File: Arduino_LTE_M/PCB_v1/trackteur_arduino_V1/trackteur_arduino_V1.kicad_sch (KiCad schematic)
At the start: 17 parts, among them J1 rPi_HDR, J2 DC/DC, J3 BATT_CAR, J4 MicroSD_Breakout, Q1 2N3904, U1 LD1117S33TR_SOT223

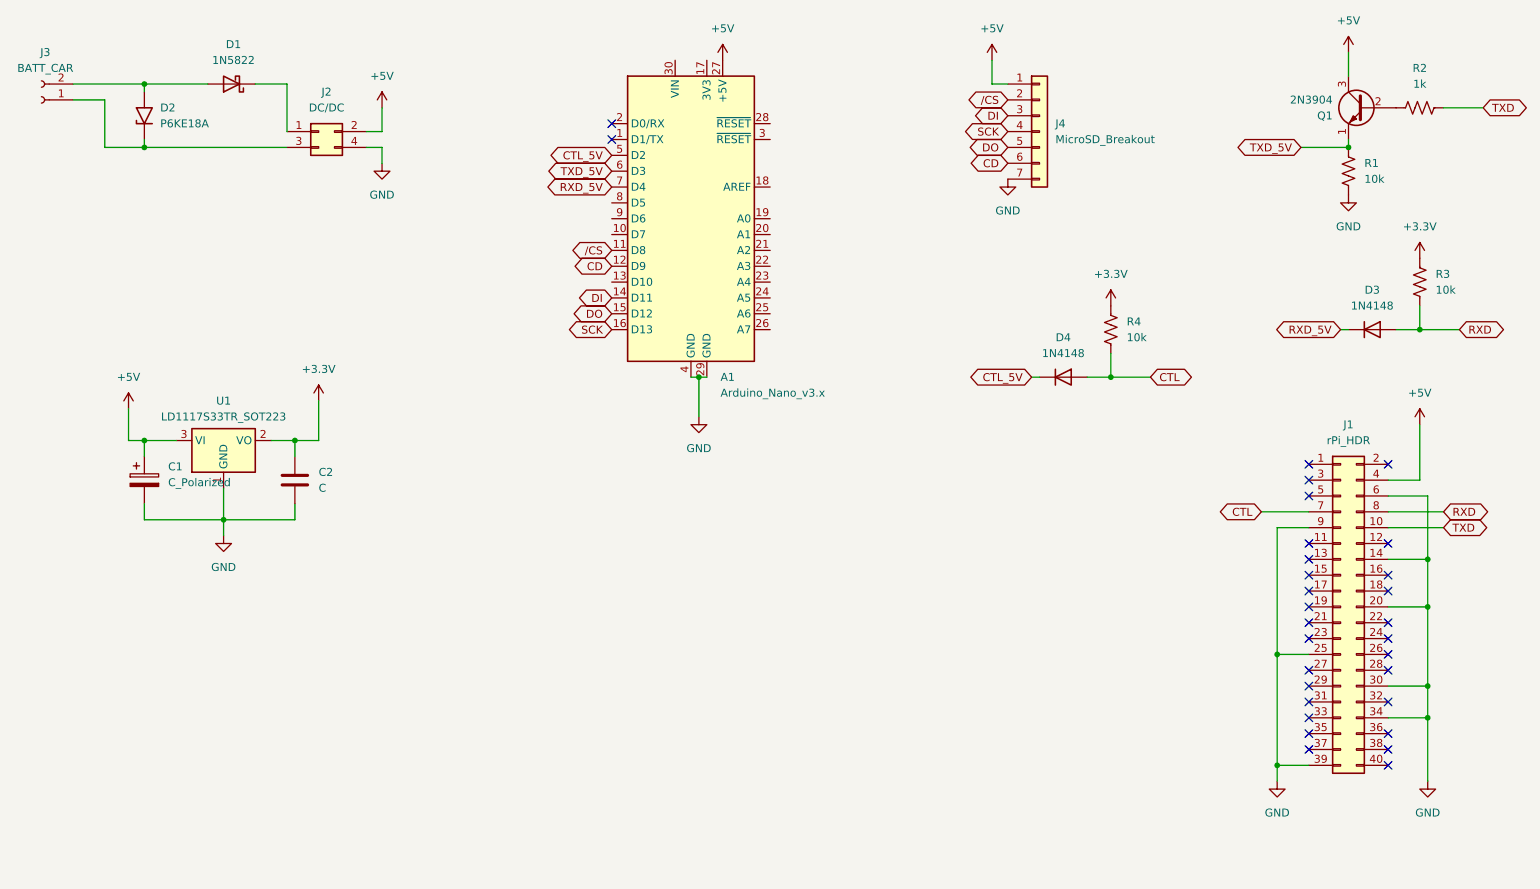
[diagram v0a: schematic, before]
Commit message: update PCB
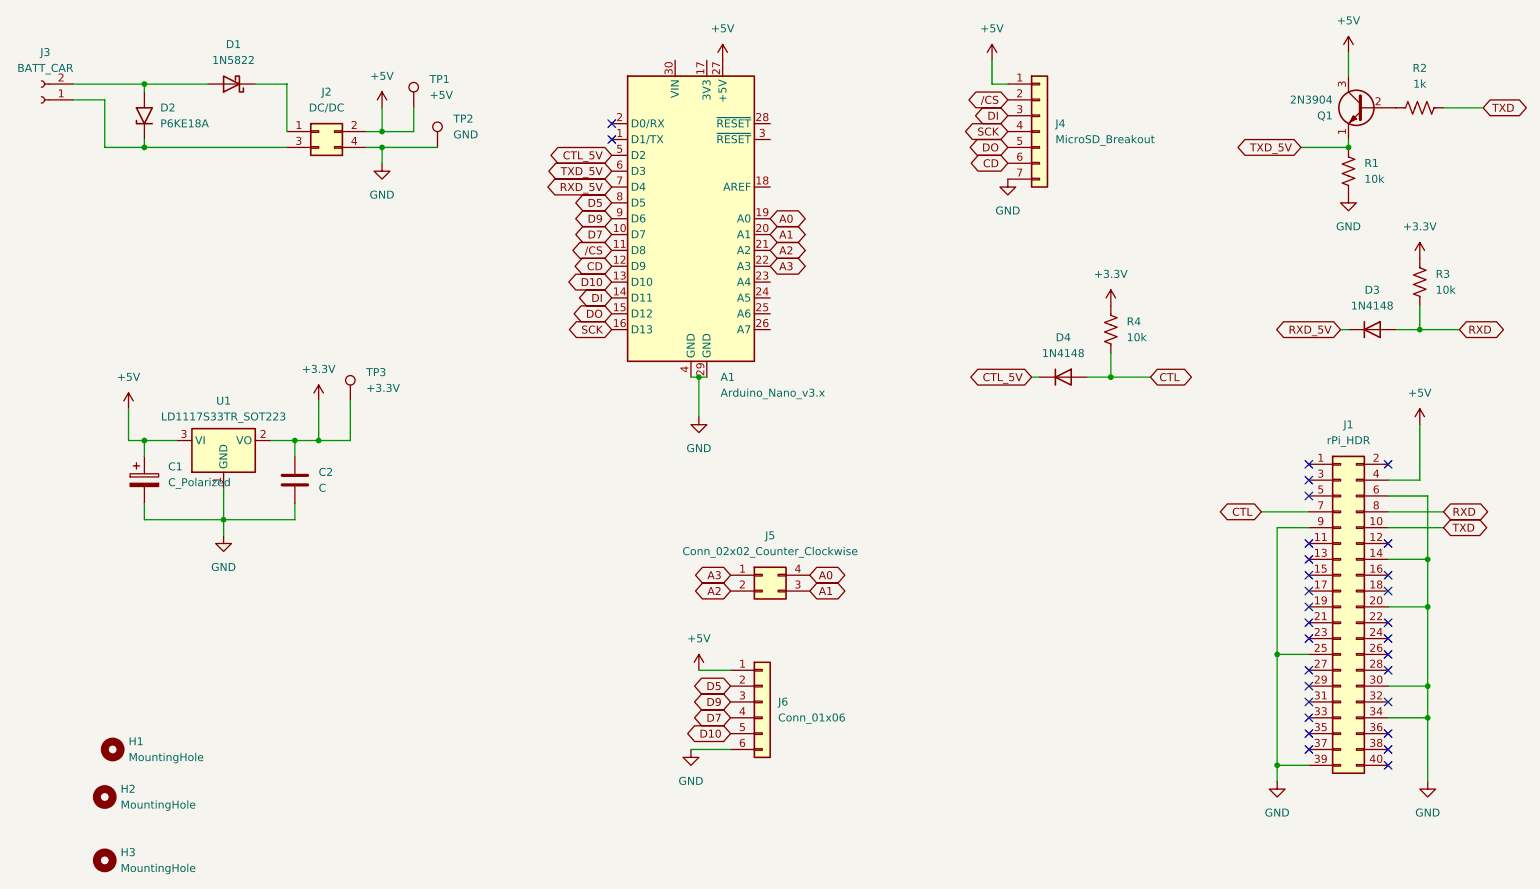
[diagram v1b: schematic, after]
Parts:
- added H1, H2, H3: MountingHole, MountingHole:MountingHole_2.7mm_M2.5, symbol Mechanical:MountingHole
- added J5: Conn_02x02_Counter_Clockwise, Connector_PinHeader_2.54mm:PinHeader_2x02_P2.54mm_Vertical, symbol Connector_Generic:Conn_02x02_Counter_Clockwise
- added J6: Conn_01x06, Connector_PinHeader_2.54mm:PinHeader_1x06_P2.54mm_Vertical, symbol Connector_Generic:Conn_01x06
- added TP1: +5V, Connector_PinHeader_2.54mm:PinHeader_1x01_P2.54mm_Vertical, symbol Connector:TestPoint
- added TP2: GND, Connector_PinHeader_2.54mm:PinHeader_1x01_P2.54mm_Vertical, symbol Connector:TestPoint
- added TP3: +3.3V, Connector_PinHeader_2.54mm:PinHeader_1x01_P2.54mm_Vertical, symbol Connector:TestPoint
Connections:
- net +3.3V: now also TP3.1
- net +5V: now also J6.1 (Pin_1), TP1.1
- net GND: now also J6.6 (Pin_6), TP2.1
- net D7: now reaches A1.10 (D7)
- net D7: now also J6.4 (Pin_4)
- net D10: now reaches A1.13 (D10)
- net D10: now also J6.5 (Pin_5)
- net A0: now reaches A1.19 (A0)
- net A0: now also J5.4 (Pin_4)
- net A1: now reaches A1.20 (A1)
- net A1: now also J5.3 (Pin_3)
- net A2: now reaches A1.21 (A2)
- net A2: now also J5.2 (Pin_2)
- net A3: now reaches A1.22 (A3)
- net A3: now also J5.1 (Pin_1)
- net D5: now reaches A1.8 (D5)
- net D5: now also J6.2 (Pin_2)
- net D9: now reaches A1.9 (D6)
- net D9: now also J6.3 (Pin_3)

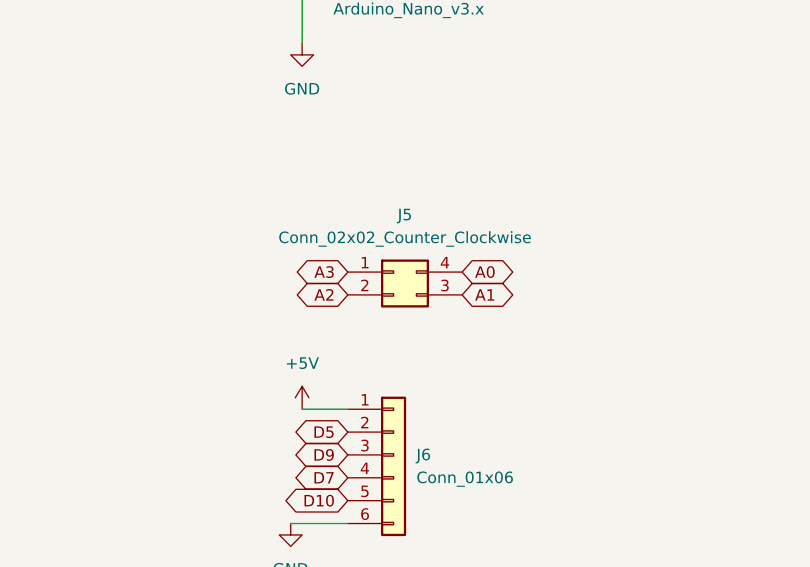
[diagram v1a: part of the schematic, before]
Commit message: Fichiers de fabrication
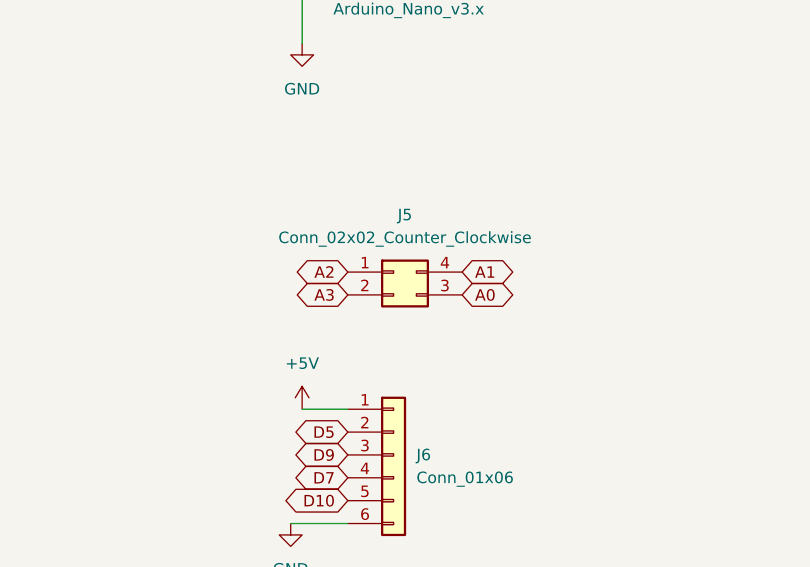
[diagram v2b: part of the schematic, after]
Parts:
- J3: footprint Connector_Wire:SolderWire-0.75sqmm_1x02_P7mm_D1.25mm_OD3.5mm -> Connector_Wire:SolderWire-2.5sqmm_1x02_P7.2mm_D2.4mm_OD3.6mm
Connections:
- net A0: now also J5.3 (Pin_3); no longer J5.4 (Pin_4)
- net A1: now also J5.4 (Pin_4); no longer J5.3 (Pin_3)
- net A2: now also J5.1 (Pin_1); no longer J5.2 (Pin_2)
- net A3: now also J5.2 (Pin_2); no longer J5.1 (Pin_1)
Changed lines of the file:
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@@
     )
   )
-  (global_label "A2" (shape bidirectional) (at 137.16 120.65 180) (fields_autoplaced)
+  (global_label "A3" (shape bidirectional) (at 137.16 120.65 180) (fields_autoplaced)
     (effects (font (size 1.27 1.27)) (justify right))
     (property "Intersheetrefs" "${INTERSHEET_REFS}" (at 130.7654 120.65 0)
@@
     )
   )
-  (global_label "A3" (shape bidirectional) (at 137.16 118.11 180) (fields_autoplaced)
+  (global_label "A2" (shape bidirectional) (at 137.16 118.11 180) (fields_autoplaced)
     (effects (font (size 1.27 1.27)) (justify right))
     (property "Intersheetrefs" "${INTERSHEET_REFS}" (at 130.7654 118.11 0)
@@
     )
   )
-  (global_label "A0" (shape bidirectional) (at 149.86 118.11 0) (fields_autoplaced)
+  (global_label "A1" (shape bidirectional) (at 149.86 118.11 0) (fields_autoplaced)
     (effects (font (size 1.27 1.27)) (justify left))
     (property "Intersheetrefs" "${INTERSHEET_REFS}" (at 156.2546 118.11 0)
@@
     )
   )
-  (global_label "A1" (shape bidirectional) (at 149.86 120.65 0) (fields_autoplaced)
+  (global_label "A0" (shape bidirectional) (at 149.86 120.65 0) (fields_autoplaced)
     (effects (font (size 1.27 1.27)) (justify left))
     (property "Intersheetrefs" "${INTERSHEET_REFS}" (at 156.2546 120.65 0)
@@
       (effects (font (size 1.27 1.27)))
     )
-    (property "Footprint" "Connector_Wire:SolderWire-0.75sqmm_1x02_P7mm_D1.25mm_OD3.5mm" (at 26.67 41.91 0)
-      (effects (font (size 1.27 1.27)) hide)
-    )
+    (property "Footprint" "Connector_Wire:SolderWire-2.5sqmm_1x02_P7.2mm_D2.4mm_OD3.6mm" (at 26.67 41.91 0)
+      (effects (font (size 1.27 1.27)) hide)
+    )
